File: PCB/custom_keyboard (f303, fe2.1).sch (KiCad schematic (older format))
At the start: 423 parts, among them IC1 FE2.1, J2 Conn_01x03_Male, J5 AVR-ISP-6, Q1 DTC123J, SW1 SW_Push, U1 24LC02BT-I/SN, U10 PRTR5V0U2X, U11 XC6206P332MR, U12 74LVC1G34, U13 XC6206P332MR, U2 PRTR5V0U2X, U3 PRTR5V0U2X, U4 PRTR5V0U2X, U5 PRTR5V0U2X, U6 PRTR5V0U2X, U7 PRTR5V0U2X, U8 PRTR5V0U2X, U9 STM32F303CBT6, Y1 8MHz, Y2 32.768KHz, Y3 12MHz

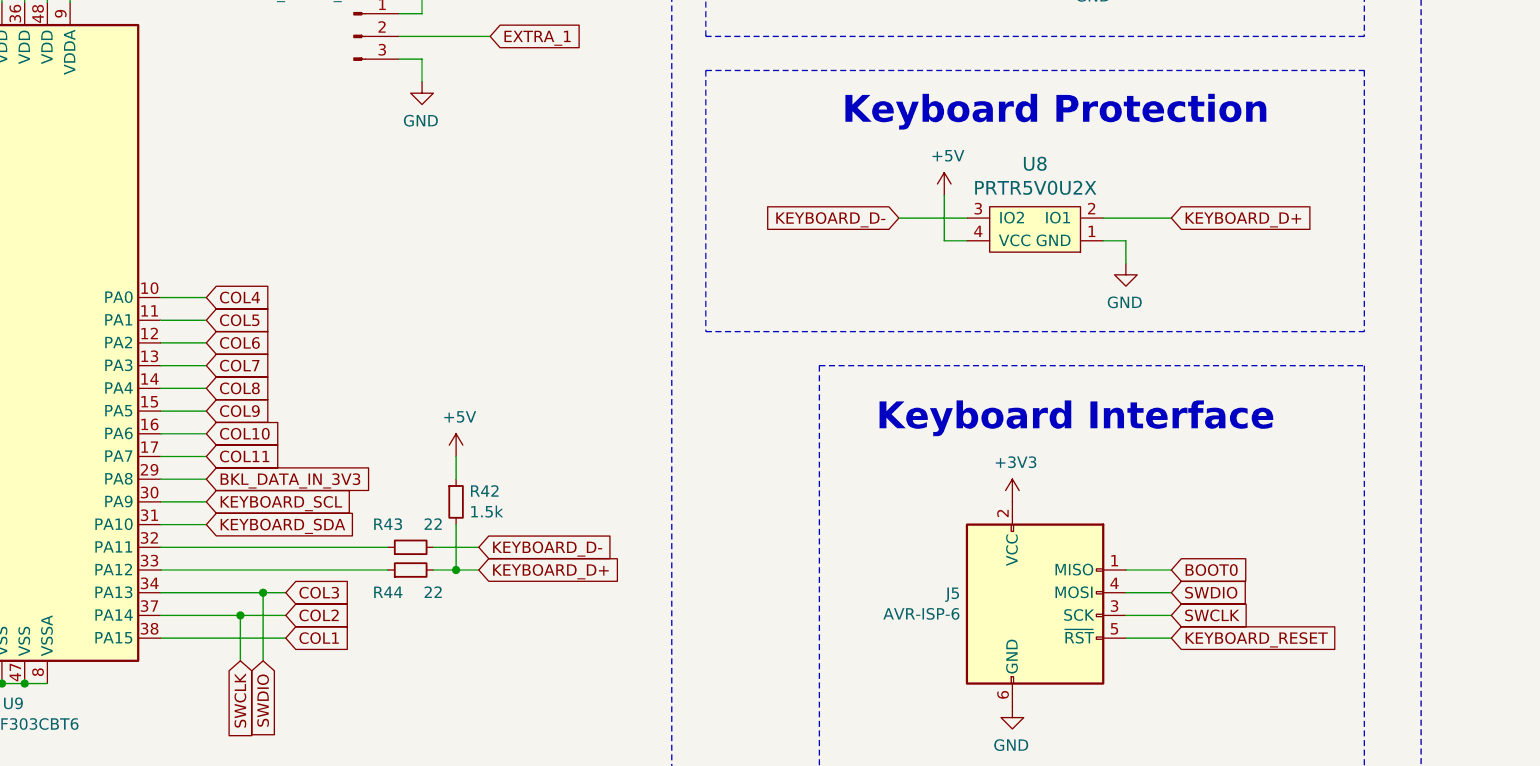
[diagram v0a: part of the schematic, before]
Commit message: Updated files, prepped for review
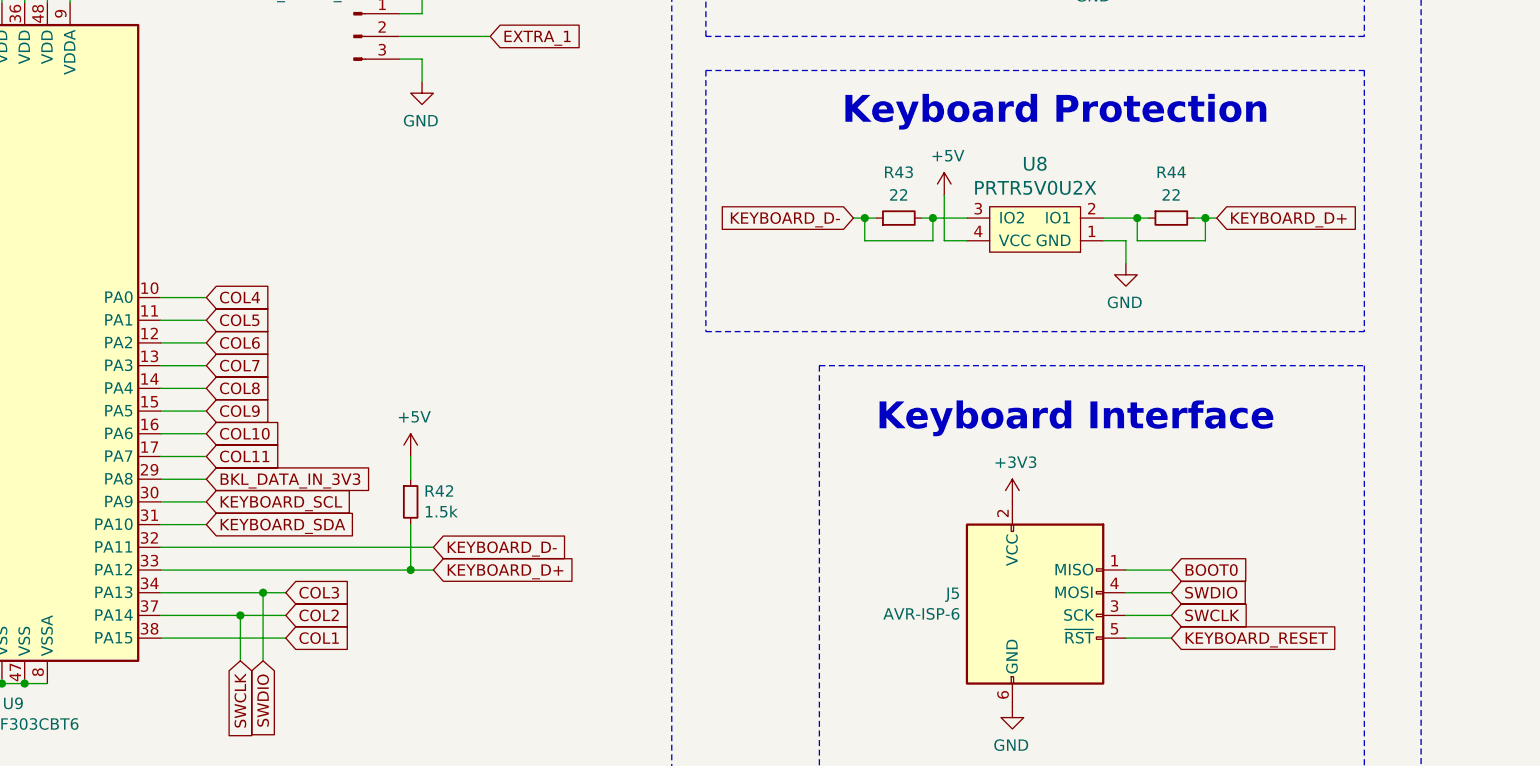
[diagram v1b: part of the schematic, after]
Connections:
- net KEYBOARD_D+: now also R44.1, U9.33 (PA12)
- net KEYBOARD_D-: now also R43.1, U9.32 (PA11)
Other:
- moved on the sheet: R42, R43, R44
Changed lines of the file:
@@
 L Device:R_Small R44
 U 1 1 83FFF6BA
-P 7250 18650
-F 0 "R44" V 7150 18750 50  0000 C CNN
-F 1 "22" V 7150 18550 50  0000 C CNN
-F 2 "Resistor_SMD:R_0805_2012Metric" H 7250 18650 50  0001 C CNN
-F 3 "~" H 7250 18650 50  0001 C CNN
-	1    7250 18650
-	0    -1   -1   0
+P 10600 17100
+F 0 "R44" V 10400 17100 50  0000 C CNN
+F 1 "22" V 10500 17100 50  0000 C CNN
+F 2 "Resistor_SMD:R_0805_2012Metric" H 10600 17100 50  0001 C CNN
+F 3 "~" H 10600 17100 50  0001 C CNN
+	1    10600 17100
+	0    -1   1    0
 $EndComp
 $Comp
 L Device:R_Small R43
 U 1 1 840036CC
-P 7250 18550
-F 0 "R43" V 7350 18650 50  0000 C CNN
-F 1 "22" V 7350 18450 50  0000 C CNN
-F 2 "Resistor_SMD:R_0805_2012Metric" H 7250 18550 50  0001 C CNN
-F 3 "~" H 7250 18550 50  0001 C CNN
-	1    7250 18550
+P 9400 17100
+F 0 "R43" V 9600 17100 50  0000 C CNN
+F 1 "22" V 9500 17100 50  0000 C CNN
+F 2 "Resistor_SMD:R_0805_2012Metric" H 9400 17100 50  0001 C CNN
+F 3 "~" H 9400 17100 50  0001 C CNN
+	1    9400 17100
 	0    -1   -1   0
 $EndComp
-Text GLabel 7550 18550 2    50   Input ~ 0
+Text GLabel 7350 18550 2    50   Input ~ 0
 KEYBOARD_D-
 Wire Wire Line
-	7450 18450 7450 18650
-Connection ~ 7450 18650
+	7250 18450 7250 18650
+Connection ~ 7250 18650
 $Comp
 L Device:R_Small R42
 U 1 1 8482A4BE
-P 7450 18350
-F 0 "R42" H 7509 18396 50  0000 L CNN
-F 1 "1.5k" H 7509 18305 50  0000 L CNN
-F 2 "Resistor_SMD:R_0805_2012Metric" H 7450 18350 50  0001 C CNN
-F 3 "~" H 7450 18350 50  0001 C CNN
-	1    7450 18350
+P 7250 18350
+F 0 "R42" H 7309 18396 50  0000 L CNN
+F 1 "1.5k" H 7309 18305 50  0000 L CNN
+F 2 "Resistor_SMD:R_0805_2012Metric" H 7250 18350 50  0001 C CNN
+F 3 "~" H 7250 18350 50  0001 C CNN
+	1    7250 18350
 	1    0    0    -1
 $EndComp
 Wire Wire Line
-	7450 18150 7450 18250
+	7250 18150 7250 18250
 $Comp
 L power:+5V #PWR0170
 U 1 1 6DAAD363
-P 7450 18150
-F 0 "#PWR0170" H 7450 18000 50  0001 C CNN
-F 1 "+5V" H 7465 18323 50  0000 C CNN
-F 2 "" H 7450 18150 50  0001 C CNN
-F 3 "" H 7450 18150 50  0001 C CNN
-	1    7450 18150
+P 7250 18150
+F 0 "#PWR0170" H 7250 18000 50  0001 C CNN
+F 1 "+5V" H 7265 18323 50  0000 C CNN
+F 2 "" H 7250 18150 50  0001 C CNN
+F 3 "" H 7250 18150 50  0001 C CNN
+	1    7250 18150
 	1    0    0    -1
 $EndComp
@@
 	7650 21050 7450 21050
 Wire Wire Line
-	7350 18550 7550 18550
-Wire Wire Line
-	7450 18650 7550 18650
-Text GLabel 10600 17100 2    50   Input ~ 0
+	7250 18650 7350 18650
+Text GLabel 10800 17100 2    50   Input ~ 0
 KEYBOARD_D+
-Text GLabel 9400 17100 0    50   Input ~ 0
-KEYBOARD_D-
 $Comp
 L power:GND #PWR0190
@@
 Wire Notes Line
 	8550 16450 11450 16450
-Wire Wire Line
-	7350 18650 7450 18650
-Wire Wire Line
-	6150 18550 7150 18550
-Wire Wire Line
-	6150 18650 7150 18650
 Text GLabel 6950 3100 1    50   Input ~ 0
 COL2
@@
 Wire Wire Line
 	10900 13200 10900 13500
-Text GLabel 7550 18650 2    50   Input ~ 0
+Text GLabel 7350 18650 2    50   Input ~ 0
 KEYBOARD_D+
 Wire Wire Line
@@
 	10400 17200 10300 17200
 Wire Wire Line
-	10300 17100 10600 17100
-Wire Wire Line
-	9400 17100 9700 17100
+	10300 17100 10450 17100
 Wire Wire Line
 	10400 17300 10400 17200
@@
 Wire Wire Line
 	15150 11550 15450 11550
+Wire Wire Line
+	6150 18550 7350 18550
+Wire Wire Line
+	6150 18650 7250 18650
+Text GLabel 9200 17100 0    50   Input ~ 0
+KEYBOARD_D-
+Wire Wire Line
+	9500 17100 9550 17100
+Wire Wire Line
+	10700 17100 10750 17100
+Wire Wire Line
+	10750 17100 10750 17200
+Wire Wire Line
+	10750 17200 10450 17200
+Wire Wire Line
+	10450 17200 10450 17100
+Connection ~ 10750 17100
+Wire Wire Line
+	10750 17100 10800 17100
+Connection ~ 10450 17100
+Wire Wire Line
+	10450 17100 10500 17100
+Wire Wire Line
+	9200 17100 9250 17100
+Wire Wire Line
+	9250 17100 9250 17200
+Wire Wire Line
+	9250 17200 9550 17200
+Wire Wire Line
+	9550 17200 9550 17100
+Connection ~ 9250 17100
+Wire Wire Line
+	9250 17100 9300 17100
+Connection ~ 9550 17100
+Wire Wire Line
+	9550 17100 9700 17100
 $EndSCHEMATC
